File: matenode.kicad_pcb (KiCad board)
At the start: 2 copper layers, 76 x 22 mm, 106 parts, among them J1 USB_C_Receptacle, J10 BAT_CONN, J2 VIN, J3 QWIIC, J4 VIN, J5 Lichtenprog_conn, J6 VIN, J7 VIN, J8 VIN, J9 SPK_OUT, Q1 MMBT2222A, Q2 MMBT2222A, Q3 BSS84, Q4 MMBT2222A, SW2 RST, SW3 B2, SW4 BOOT/B1, U1 SPX3819M5-L-3-3, U2 BQ24073RGT, U3 JLC_OLED, U4 ESP32-C3-WROOM-02, U5 PAM8302AAD

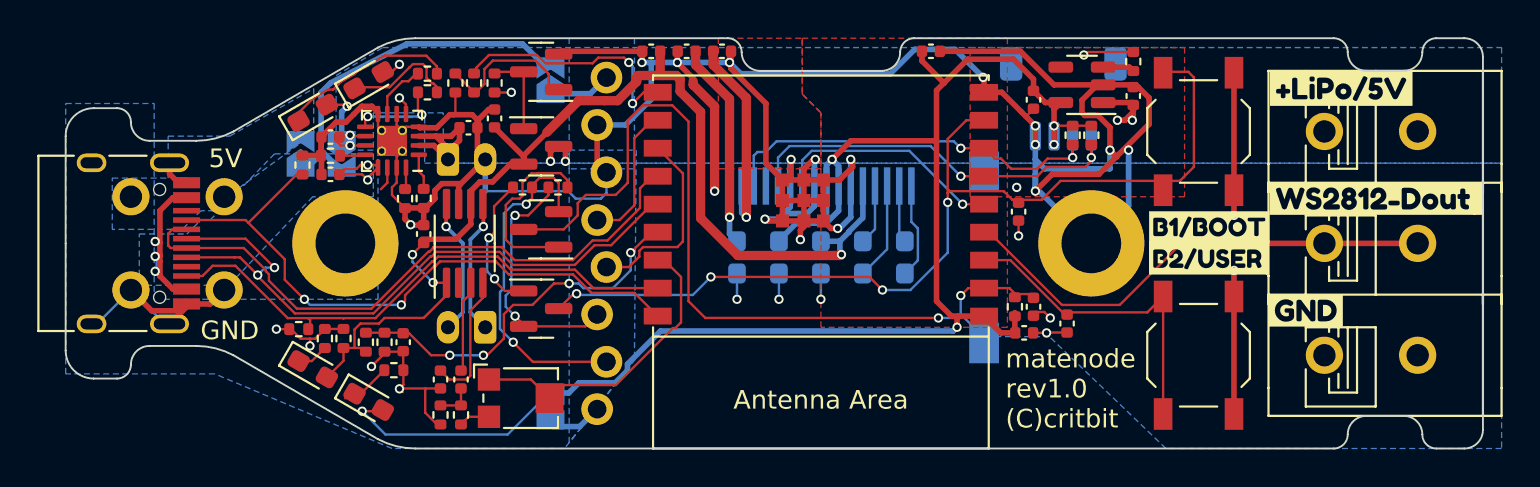
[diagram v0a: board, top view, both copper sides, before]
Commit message: final final
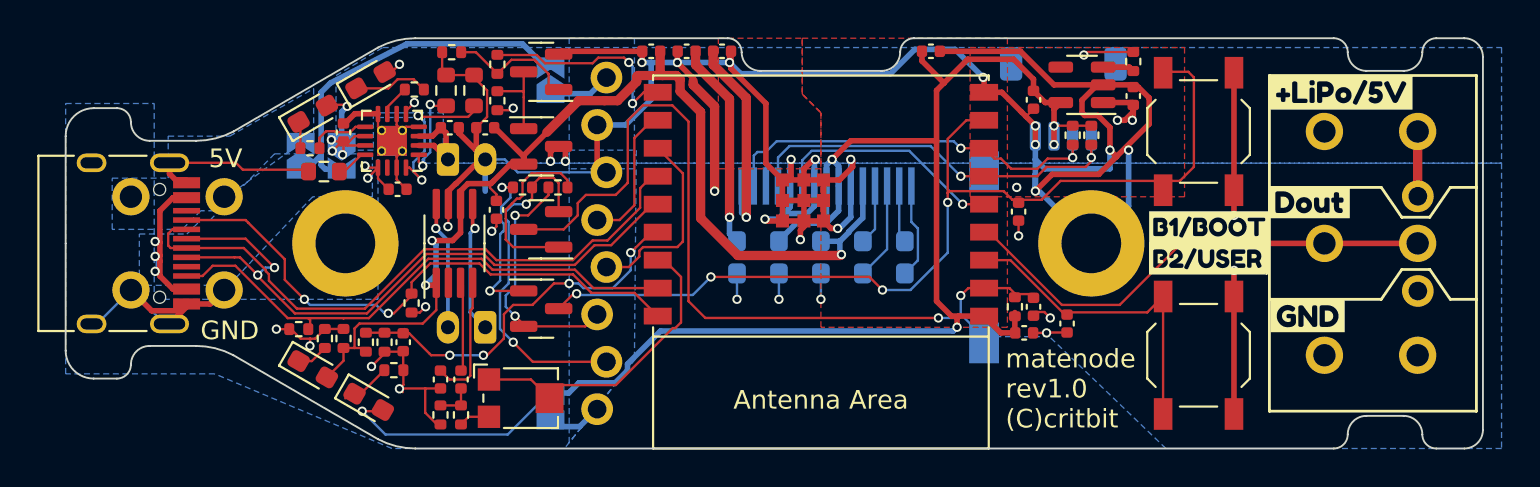
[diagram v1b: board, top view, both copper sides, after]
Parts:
- removed kibuzzard-6394CBFF (x2): G***, kibuzzard-6394CBFF
- added J11: 2.54 header, Connector_PinHeader_2.54mm:PinHeader_1x03_P2.54mm_Vertical, F.Cu at (128.0, 78.5)
- added kibuzzard-63966DAE: G***, kibuzzard-63966DAE, F.Cu at (122.2, 78.8)
- added kibuzzard-63966DAE: G***, kibuzzard-63966DAE, B.Cu at (122.3, 78.9)
- J4: value VIN -> Vout
- J7: value VIN -> Dout
- J8: value VIN -> Gout
- R12, R13, R14: footprint Resistor_SMD:R_0402_1005Metric -> Resistor_SMD:R_0603_1608Metric
- moved R1 9.43 mm to (74.0, 84.2), turned to -90 degrees
- moved kibuzzard-6394CC15 7.10 mm to (122.1, 84.8)
- moved R7 6.98 mm to (68.6, 75.9), turned to 180 degrees
- moved R13 6.88 mm to (77.4, 72.8), turned to -90 degrees
- moved R14 5.91 mm to (75.9, 72.8), turned to -90 degrees
- moved C17 4.11 mm to (78.6, 79.2), turned to -90 degrees
- moved C3 3.69 mm to (73.3, 78.1), turned to 0 degrees
- moved D1 3.56 mm to (71.8, 72.2)
- moved D2 3.50 mm to (68.8, 74.0)
- moved kibuzzard-6394CBE8 3.41 mm to (123.9, 73.0)
- moved R25 1.66 mm to (76.2, 70.8), turned to 180 degrees
- moved R24 1.60 mm to (78.7, 71.4)
- moved R6 1.10 mm to (74.2, 72.8)
- moved C19 1.00 mm to (76.1, 74.8)
- moved R15 0.96 mm to (78.7, 73.3)
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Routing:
- net Net-(R13-Pad2): track 1.17 -> 8.63 mm, vias 0 -> 2
- net Net-(D1-Pad1): track 9.37 -> 4.05 mm
- net +4V: track 18.4 -> 23.0 mm, vias 11 -> 12
- net Net-(D2-Pad1): track 6.04 -> 1.45 mm
- net /CC1: track 34.1 -> 30.7 mm
- net Net-(R14-Pad2): track 1.94 -> 5.13 mm, vias 0 -> 2
- net Net-(C19-Pad1): track 7.72 -> 5.10 mm
- net /IO_PERIPH_ENA: track 13.1 -> 11.4 mm
- net Net-(R7-Pad1): track 4.89 -> 3.30 mm, vias 2 -> 0
- net Net-(R6-Pad1): track 3.13 -> 1.70 mm
- net Net-(Q1-Pad1): track 7.53 -> 8.95 mm
- net unconnected-(U2-Pad14): track 1.31 -> 0.00 mm
- net VBUS: track 32.9 -> 31.9 mm
- net Net-(Q4-Pad1): track 8.09 -> 7.20 mm
- net /PERIPH_ENA: track 58.7 -> 59.5 mm
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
